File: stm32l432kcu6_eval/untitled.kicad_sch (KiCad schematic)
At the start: 7 parts, among them J3 USB_C_Receptacle, U2 XC6206PxxxMR, U3 USBLC6-2SC6

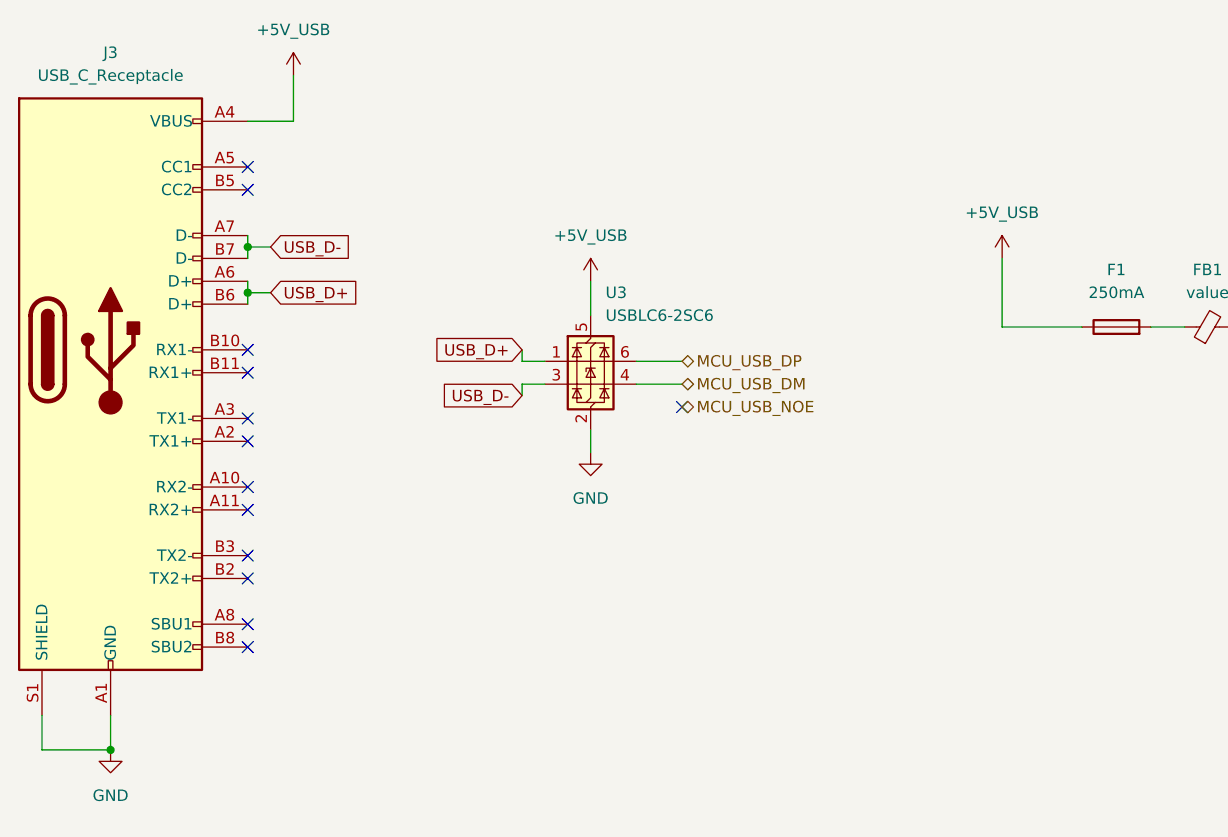
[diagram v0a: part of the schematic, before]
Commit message: pin arragment 1
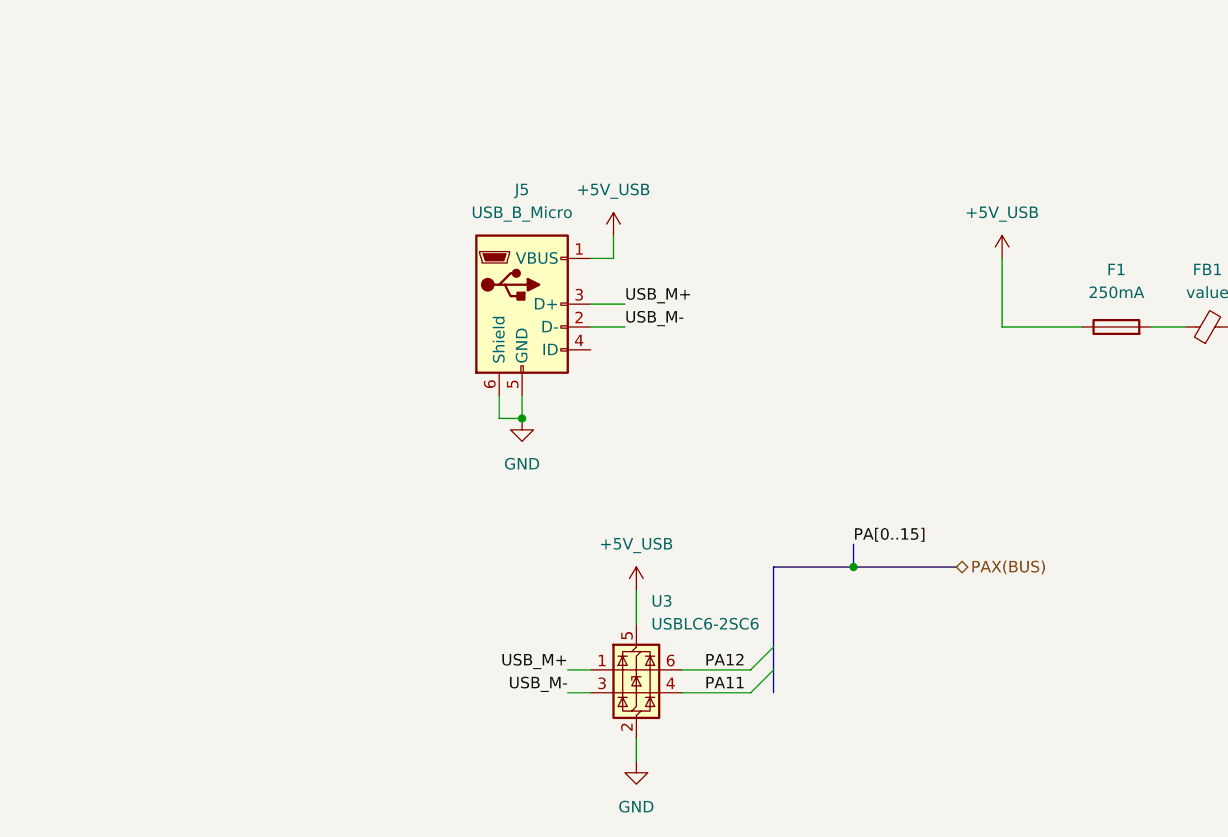
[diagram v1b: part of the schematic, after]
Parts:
- removed J3: USB_C_Receptacle, Connector_USB:USB_C_Receptacle_Molex_105450-0101, symbol Connector:USB_C_Receptacle
- added J5: USB_B_Micro, Connector_USB:USB_Micro-B_Molex-105017-0001, symbol Connector:USB_B_Micro
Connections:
- net +5V_USB: now also J5.1 (VBUS)
- net GND: now also J5.5 (GND), J5.6 (Shield)
- net MCU_USB_DM renamed PA11
- net MCU_USB_DP renamed PA12
- net USB_D+ renamed USB_M+
- net USB_M+: now also J5.3 (D+)
- net USB_D- renamed USB_M-
- net USB_M-: now also J5.2 (D-)
- no-connect marks 13 -> 0
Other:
- moved on the sheet: U3

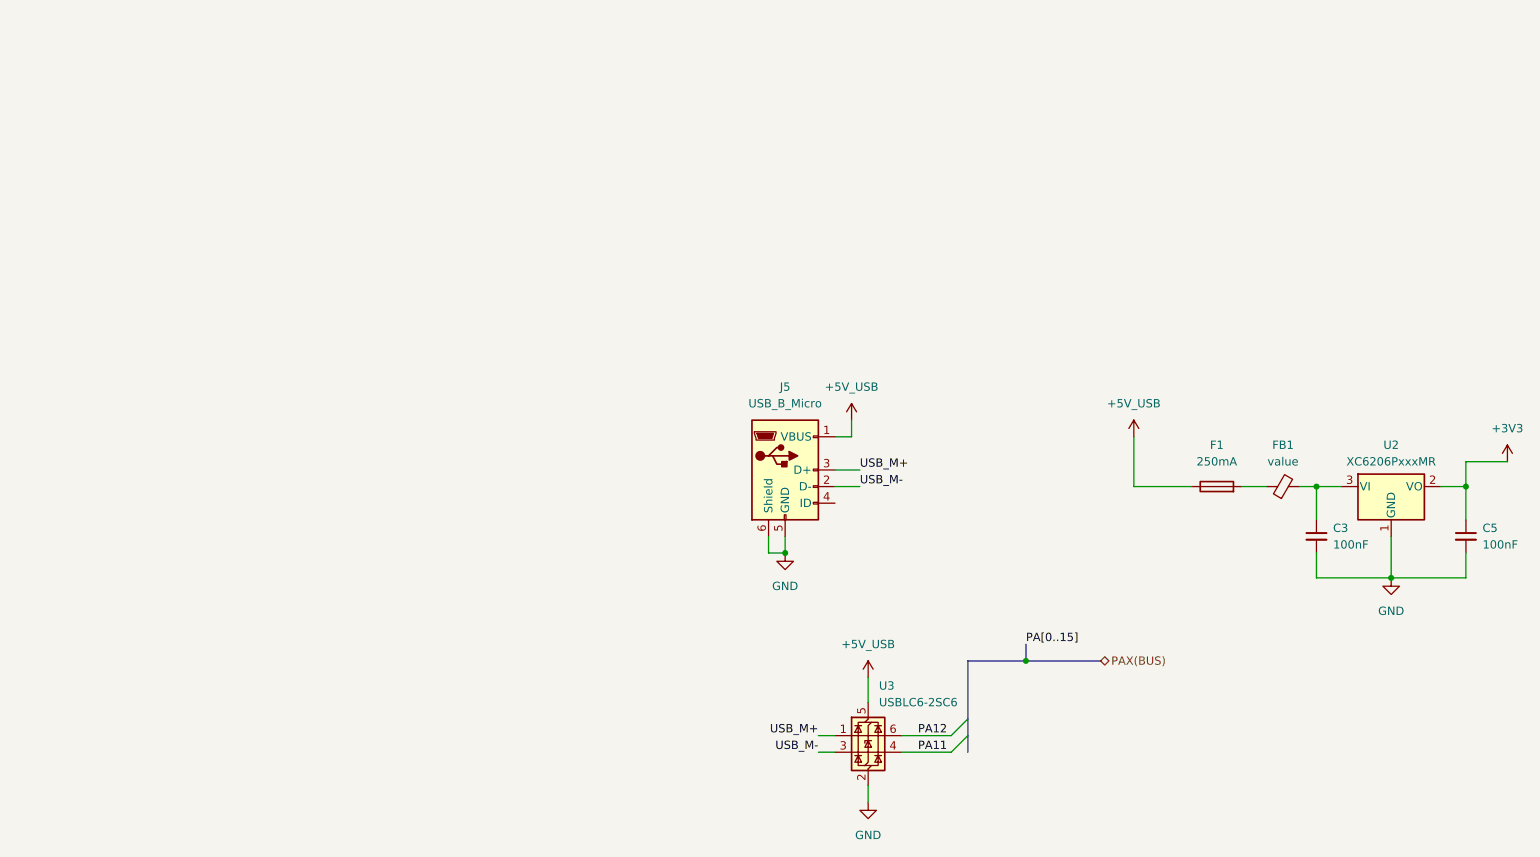
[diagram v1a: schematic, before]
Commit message: organisation save 1
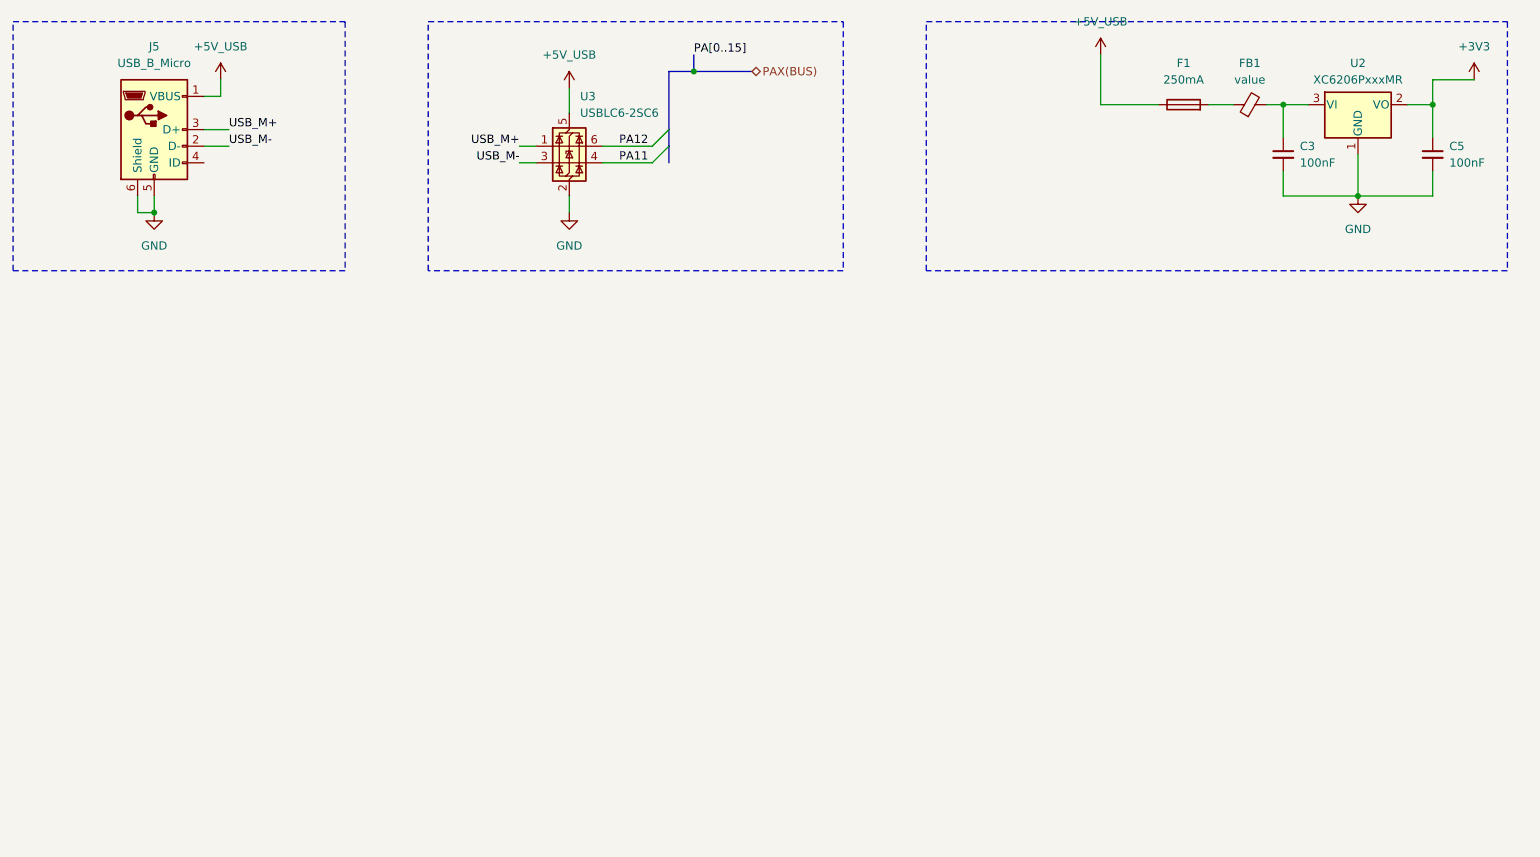
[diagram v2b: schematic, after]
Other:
- moved on the sheet: C3, C5, F1, FB1, J5, U2, U3

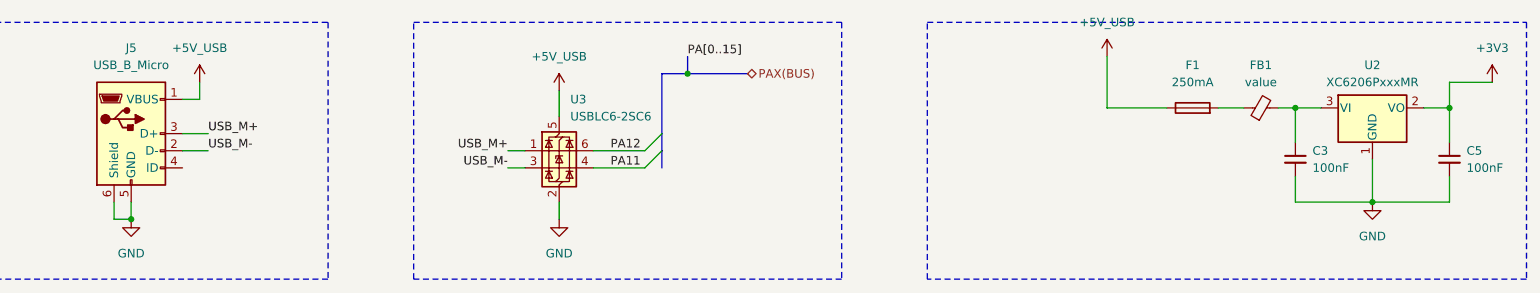
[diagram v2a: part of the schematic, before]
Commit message: organisation save 2
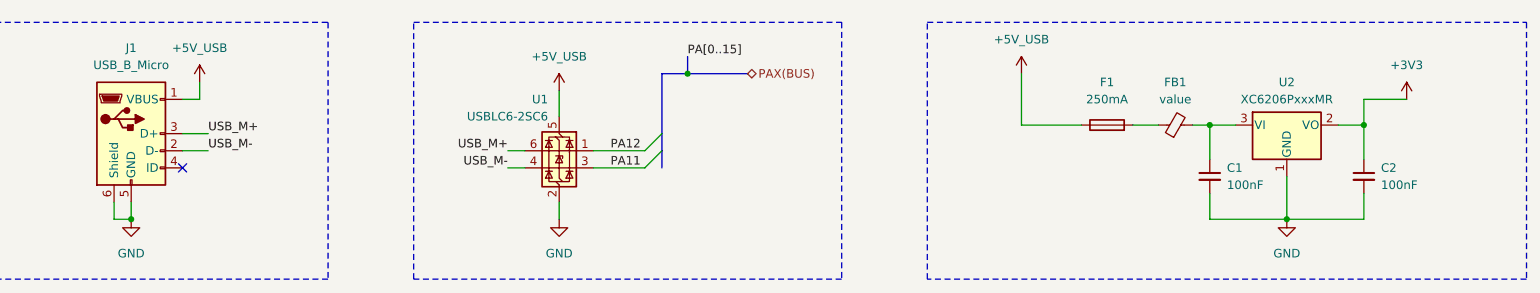
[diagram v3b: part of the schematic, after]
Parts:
- renumbered C3 to C1, C5 to C2, J5 to J1, U3 to U1
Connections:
- net PA11: now also U1.3 (I/O2); no longer U1.4 (I/O2)
- net PA12: now also U1.1 (I/O1); no longer U1.6 (I/O1)
- net USB_M+: now also U1.6 (I/O1); no longer U1.1 (I/O1)
- net USB_M-: now also U1.4 (I/O2); no longer U1.3 (I/O2)
- no-connect marks 0 -> 1
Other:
- moved on the sheet: C1, C2, F1, FB1, U2
